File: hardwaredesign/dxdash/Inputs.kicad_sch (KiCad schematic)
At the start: 30 parts, among them J2 Conn_01x06_Pin, SW2 SW_Push, SW3 SW_Push, SW4 SW_Push, SW5 SW_Push

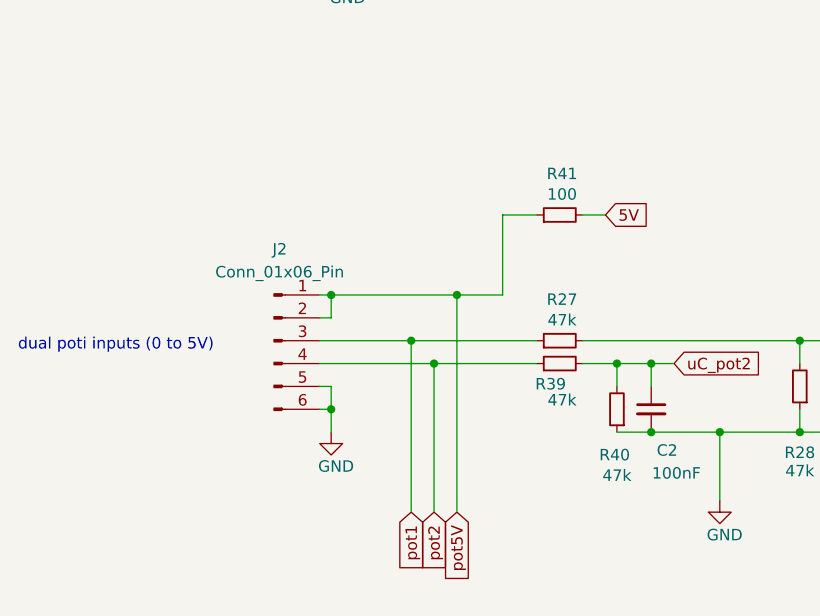
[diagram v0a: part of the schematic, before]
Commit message: more layout
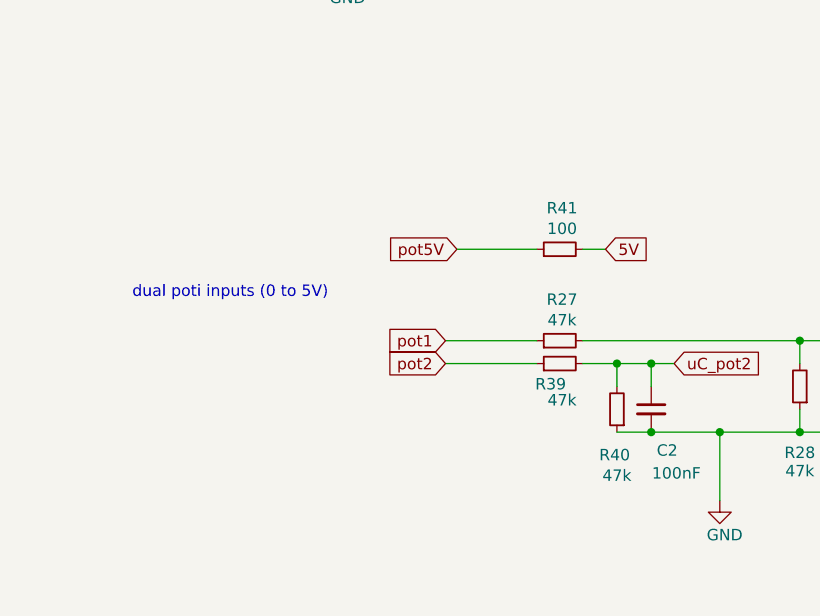
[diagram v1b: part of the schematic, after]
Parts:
- removed J2: Conn_01x06_Pin, Connector_PinHeader_2.54mm:PinHeader_1x06_P2.54mm_Vertical, symbol Connector:Conn_01x06_Pin
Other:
- moved on the sheet: R41
